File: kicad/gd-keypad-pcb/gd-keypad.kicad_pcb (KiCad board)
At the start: 2 copper layers, 152.5 x 68 mm, 61 parts, among them J2 USB_C_Receptacle_USB2.0_16P, J3 TC2030, SW1 TS-1187A-B-A-B, SW2 TS-1187A-B-A-B, SW3 RotaryEncoder_Switch_MP, U1 AT32F405RCT7, U2 USBLC6-2SC6, U3 TLV75733PDBV, U4 XC6206P332MR-G, U5 SW_MX_HE, U6 SW_MX_HE, U7 SW_MX_HE, Y1 X322512MSB4SI

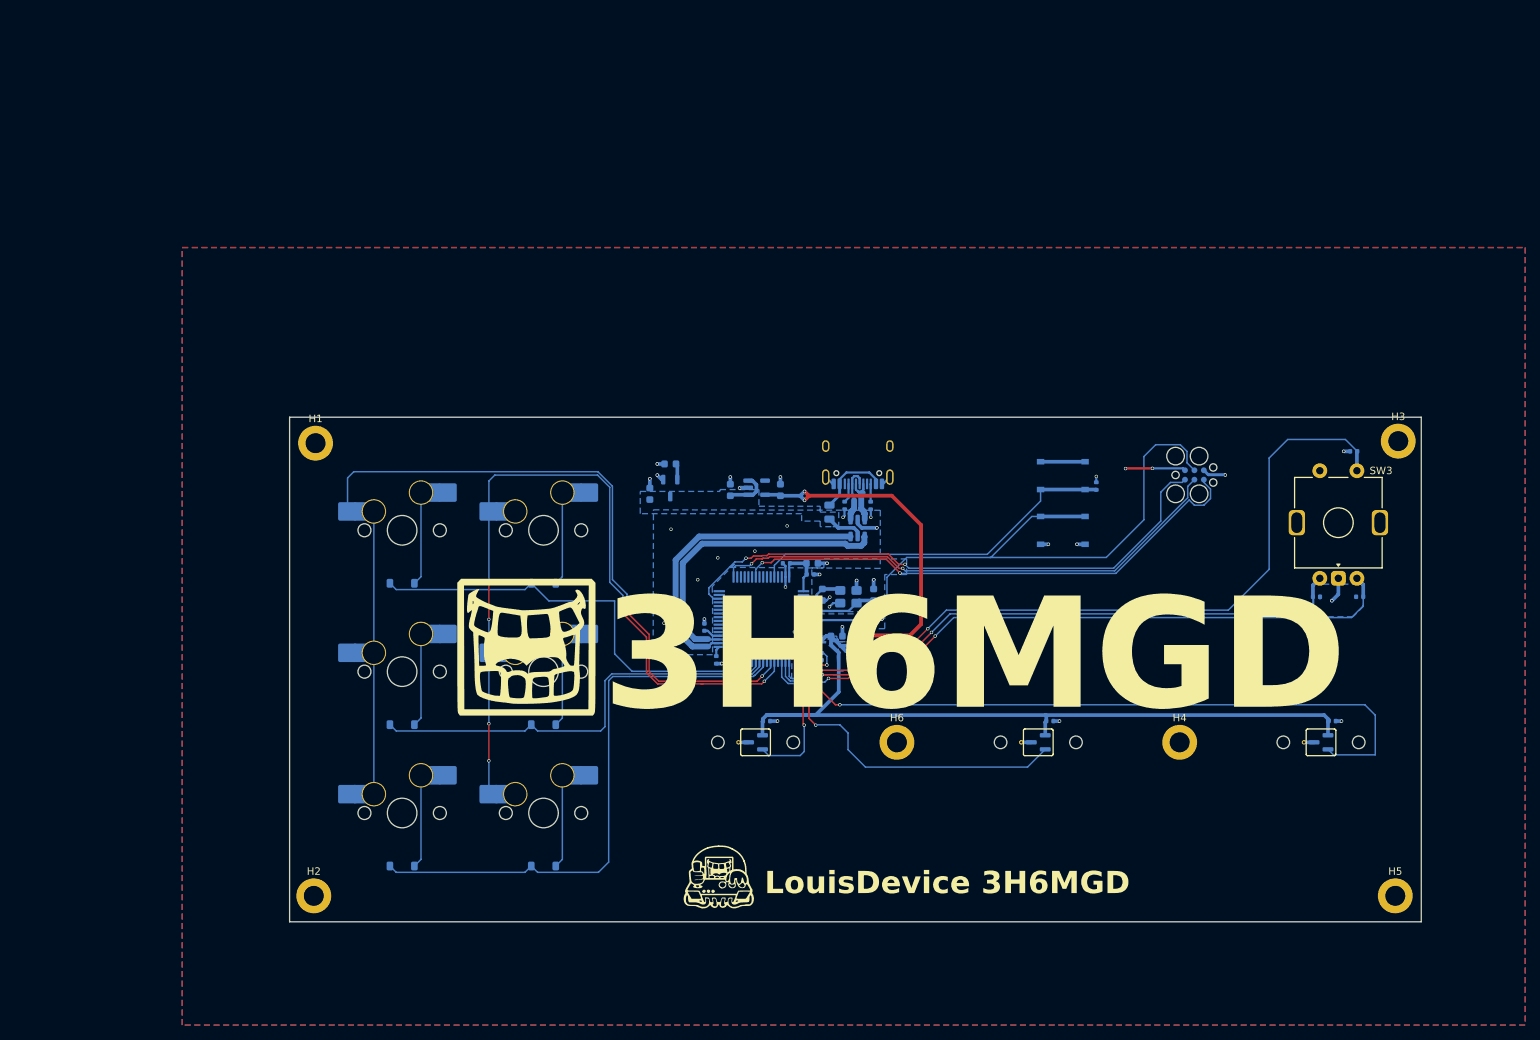
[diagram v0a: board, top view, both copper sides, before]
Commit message: updated pcb design
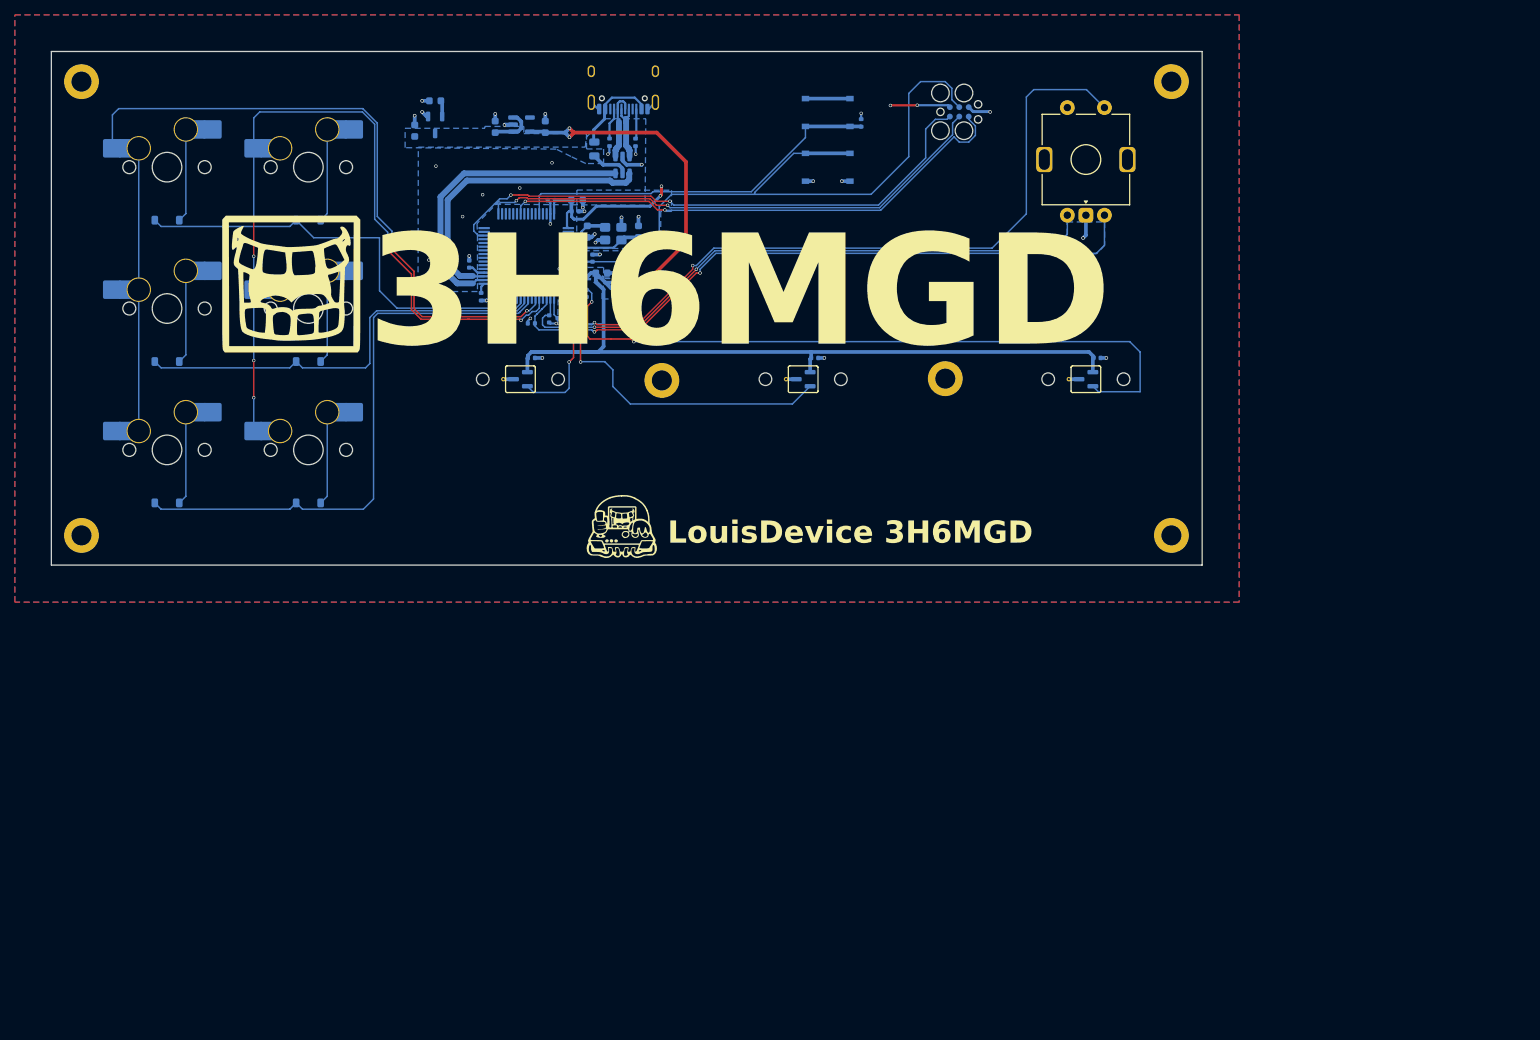
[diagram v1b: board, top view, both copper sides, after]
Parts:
- moved H3 177.9 mm to (18.0, 79.2)
- moved H2 159.4 mm to (164.9, 18.0)
- moved H5 120.8 mm to (96.2, 58.3)
- moved C7 117.5 mm to (78.6, 50.6)
- moved C8 110.0 mm to (81.0, 50.0), turned to 90 degrees
- moved C9 108.3 mm to (82.6, 49.9), turned to 0 degrees
- moved C160 61.6 mm to (86.9, 41.8), turned to 90 degrees
- moved SW3 59.6 mm to (153.3, 28.5)
- moved J2 59.6 mm to (91.0, 17.6)
- moved R4 58.3 mm to (123.1, 23.6)
- moved C1 58.3 mm to (78.6, 55.2)
- moved C148 58.3 mm to (73.8, 24.1)
- moved C149 58.3 mm to (80.5, 24.1)
- moved C150 58.3 mm to (62.9, 24.6)
- moved C3 58.3 mm to (116.8, 55.2)
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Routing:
- net +3.3V: track 28.1 -> 43.9 mm, vias 2 -> 4
- net ENCODER S1: track 104.3 -> 100.9 mm
- net USB_PLUG_D+: track 6.65 -> 9.10 mm
- net VBUS: track 10.3 -> 12.0 mm
- net Net-(J2-CC2): track 2.41 -> 4.03 mm
- net Net-(J2-CC1): track 2.61 -> 4.23 mm
- net USB_PLUG_D-: track 7.88 -> 9.42 mm
- net ENCODER A: track 81.5 -> 83.0 mm
- net ENCODER B: track 89.3 -> 90.7 mm
- net GND: track 53.4 -> 54.5 mm, vias 40 -> 42
- net NRST: track 87.7 -> 88.6 mm
- net HE SENSOR 2: track 49.0 -> 48.4 mm
- net SWO: track 71.3 -> 70.8 mm
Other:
- board size 152.5 x 68 mm -> 155.1 x 69.2 mm

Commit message: finalized pcb design
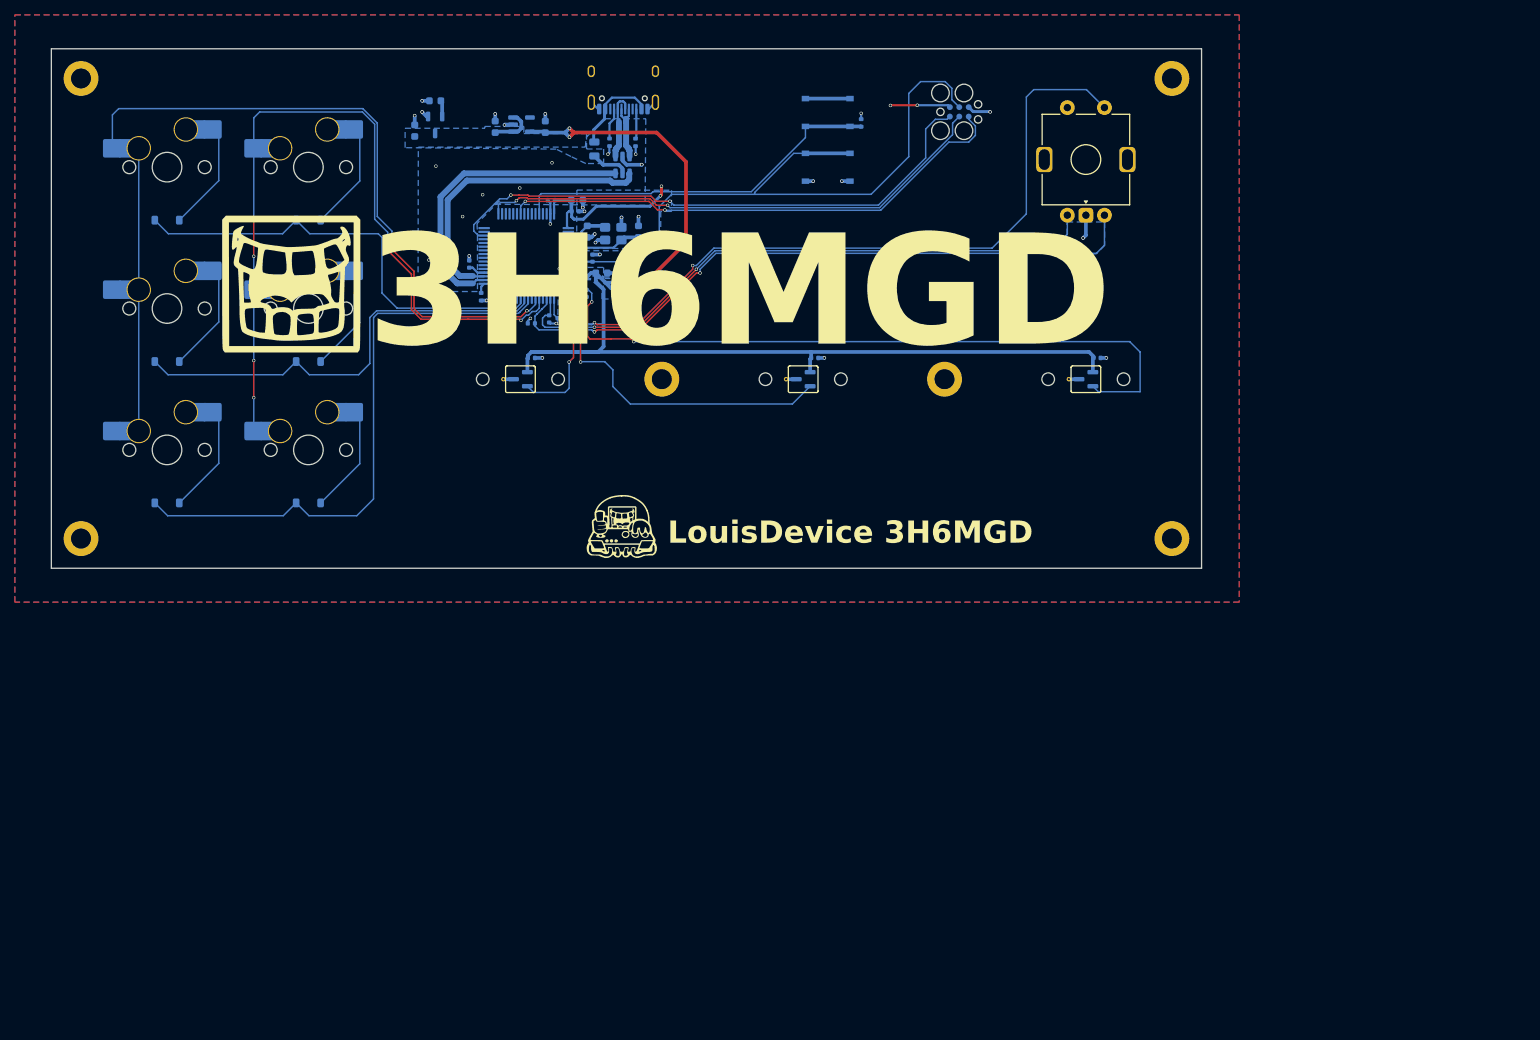
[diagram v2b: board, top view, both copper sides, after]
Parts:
- MX1, MX2, MX3, MX4, MX5, MX6: footprint PCM_marbastlib-mx:SW_MX_HS_CPG151101S11_1u -> PCM_marbastlib-mx:SW_MX_HS_KS-2P02B01-01_1u
- moved H1 0.43 mm to (17.9, 17.6)
- moved H3 0.43 mm to (17.9, 79.6)
- moved H4 0.43 mm to (164.9, 79.6)
- moved H2 0.43 mm to (164.9, 17.6)
- moved H5 0.17 mm to (96.2, 58.1)
- moved H6 0.13 mm to (134.3, 58.1)
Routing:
- net Net-(D5-A): track 12.6 -> 14.8 mm
- net Net-(D1-A): track 12.6 -> 14.8 mm
- net Net-(D3-A): track 12.6 -> 14.8 mm
- net Net-(D4-A): track 12.6 -> 14.8 mm
- net Net-(D6-A): track 12.6 -> 14.8 mm
- net Net-(D2-A): track 12.6 -> 14.8 mm
- net ROW 1: track 58.8 -> 60.4 mm
- net ROW 2: track 78.1 -> 79.5 mm
- net ROW 0: track 60.1 -> 61.1 mm
- net SWO: track 70.8 -> 70.2 mm
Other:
- board size 155.1 x 69.2 mm -> 155 x 70 mm
